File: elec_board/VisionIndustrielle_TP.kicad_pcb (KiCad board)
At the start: 2 copper layers, 148 x 111.1 mm, 48 parts, among them J1 Capt1, J10 Morpho_Gauche, J11 RN42X-DROITE, J12 BAT_IN, J13 Motor1_Out_JST, J14 Morpho_Droite, J15 Poussoir1, J16 Poussoir2, J17 Motor1_Out_Pin, J18 GND_reg, J19 V_ECLAIRAGE, J2 CFG3_Open, J20 5V_reg, J21 3.3V_reg, J22 nRF24L01, J23 V_Ecl_1, J24 V_Ecl_2, J25 V_Ecl_3, J26 Poussoir3, J27 TMC2100_A_b, J28 Motor2_Out_JST, J29 Motor2_Out_Pin, J3 Capt2, J30 TMC2100_B_b, J31 TMC2100_Vref, J32 LED Strip 1, J33 LED Strip 2, J4 Capt3, J5 VMOT, J6 TMC2100_A, J7 TMC2100_B, J8 TMC2100_Vref, J9 RN42X-GAUCHE, Q1 IRL540N, Q2 IRL540N, Q3 IRL540N, U1 L7805

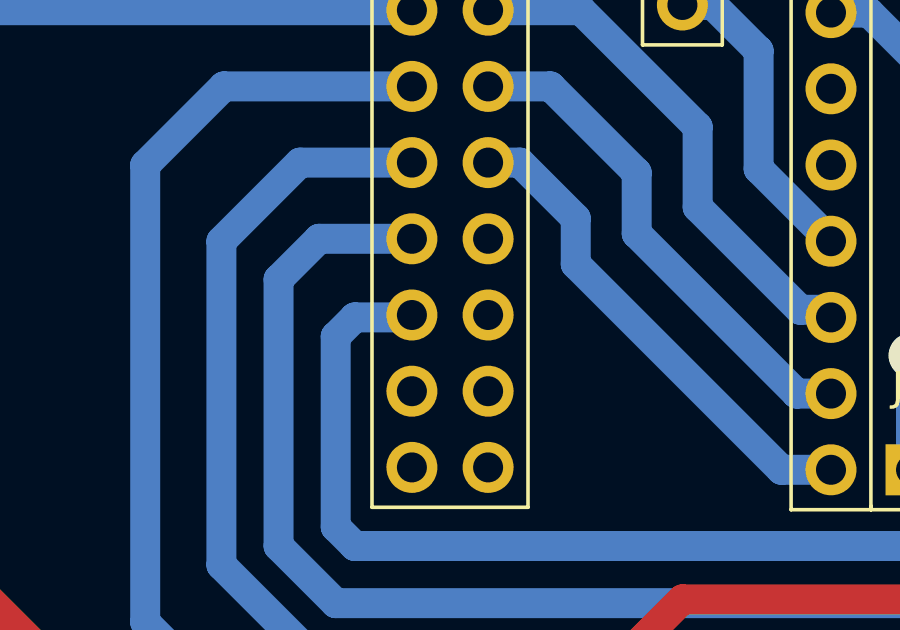
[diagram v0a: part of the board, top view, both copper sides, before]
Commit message: Update Schematic
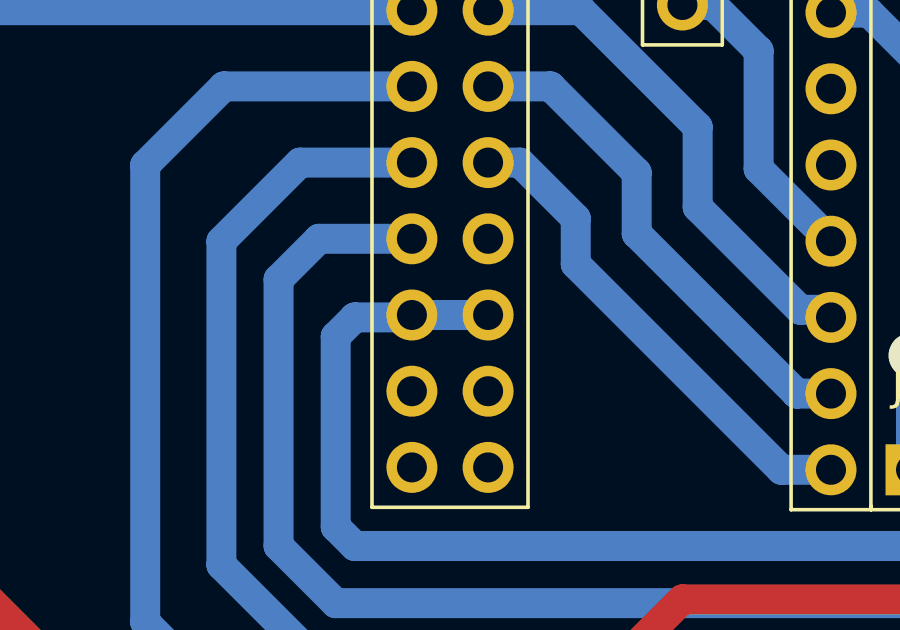
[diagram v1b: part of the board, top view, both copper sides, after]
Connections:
- J14 pad 36: Net-(J14-Pad36) -> STEP_NUC
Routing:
- net STEP_NUC: track 51.1 -> 53.6 mm
